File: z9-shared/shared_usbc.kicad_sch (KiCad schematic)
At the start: 10 parts, among them J801 USB_C_Receptacle_USB2.0_16P

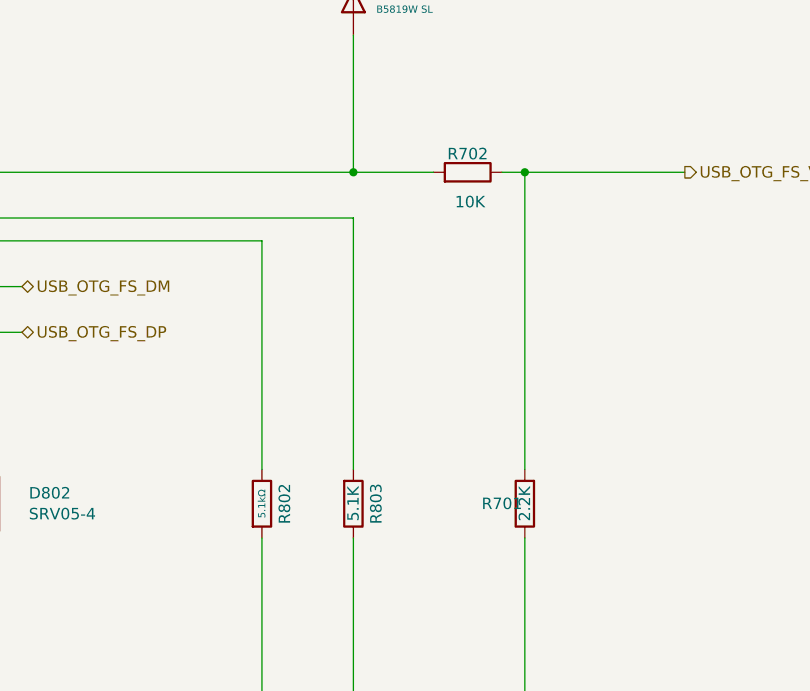
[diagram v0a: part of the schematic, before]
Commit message: pdm sch drc clean
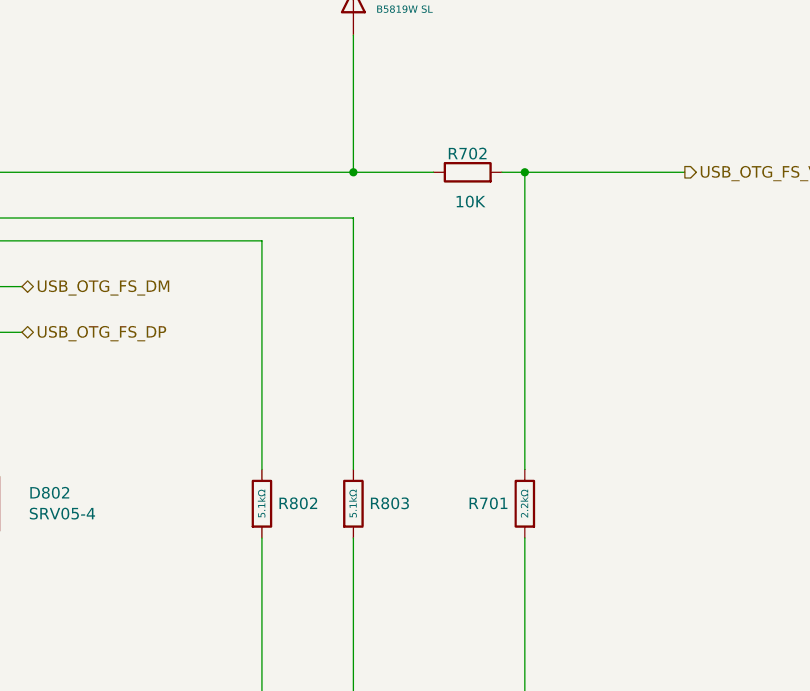
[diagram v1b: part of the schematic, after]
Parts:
- R701: value 2.2K -> 2.2kΩ; footprint (none) -> PCM_JLCPCB:R_0402; symbol Device:R -> dnt_global:Resistor_0402,2.2kΩ; Attrition Qty (none) -> 10; Category (none) -> Resistors,Chip Resistor - Surface Mount; Class (none) -> Basic Component; LCSC (none) -> C25879; Manufacturer (none) -> UNI-ROYAL(Uniroyal Elec); Minimum Qty (none) -> 20; Operating Temperature Range (none) -> -55°C~+155°C; Overload Voltage (Max) (none) -> 50V; Part (none) -> 0402WGF2201TCE; Power(Watts) (none) -> 62.5mW; Price (none) -> 0.004USD; Process (none) -> SMT; Resistance (none) -> 2.2kΩ; Stock (none) -> 1767502; Temperature Coefficient (none) -> ±100ppm/°C; Tolerance (none) -> ±1%; Type (none) -> Thick Film Resistors
- R702: footprint (none) -> PCM_JLCPCB:R_0402; symbol Device:R -> dnt_global:Resistor_0402,10kΩ; Attrition Qty (none) -> 10; Category (none) -> Resistors,Chip Resistor - Surface Mount; Class (none) -> Basic Component; LCSC (none) -> C25744; Manufacturer (none) -> UNI-ROYAL(Uniroyal Elec); Minimum Qty (none) -> 20; Operating Temperature Range (none) -> -55°C~+155°C; Overload Voltage (Max) (none) -> 50V; Part (none) -> 0402WGF1002TCE; Power(Watts) (none) -> 62.5mW; Price (none) -> 0.004USD; Process (none) -> SMT; Resistance (none) -> 10kΩ; Stock (none) -> 24372091; Temperature Coefficient (none) -> ±100ppm/°C; Tolerance (none) -> ±1%; Type (none) -> Thick Film Resistors
- R802: footprint PCM_JLCPCB:R_0603 -> PCM_JLCPCB:R_0402; symbol PCM_JLCPCB-Resistors:0603,5.1kΩ -> dnt_global:Resistor_0402,5.1kΩ; LCSC C23186 -> C25905; Overload Voltage (Max) 75V -> 50V; Part 0603WAF5101T5E -> 0402WGF5101TCE; Power(Watts) 100mW -> 62.5mW; Stock 9223405 -> 3534773
- R803: value 5.1K -> 5.1kΩ; footprint (none) -> PCM_JLCPCB:R_0402; symbol Device:R -> dnt_global:Resistor_0402,5.1kΩ; Attrition Qty (none) -> 10; Category (none) -> Resistors,Chip Resistor - Surface Mount; Class (none) -> Basic Component; LCSC (none) -> C25905; Manufacturer (none) -> UNI-ROYAL(Uniroyal Elec); Minimum Qty (none) -> 20; Operating Temperature Range (none) -> -55°C~+155°C; Overload Voltage (Max) (none) -> 50V; Part (none) -> 0402WGF5101TCE; Power(Watts) (none) -> 62.5mW; Price (none) -> 0.004USD; Process (none) -> SMT; Resistance (none) -> 5.1kΩ; Stock (none) -> 3534773; Temperature Coefficient (none) -> ±100ppm/°C; Tolerance (none) -> ±1%; Type (none) -> Thick Film Resistors
